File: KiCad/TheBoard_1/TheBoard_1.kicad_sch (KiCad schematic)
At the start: 27 parts, among them U1 TL431D, U2 TL431D, U4 TL431D, U5 TL431D

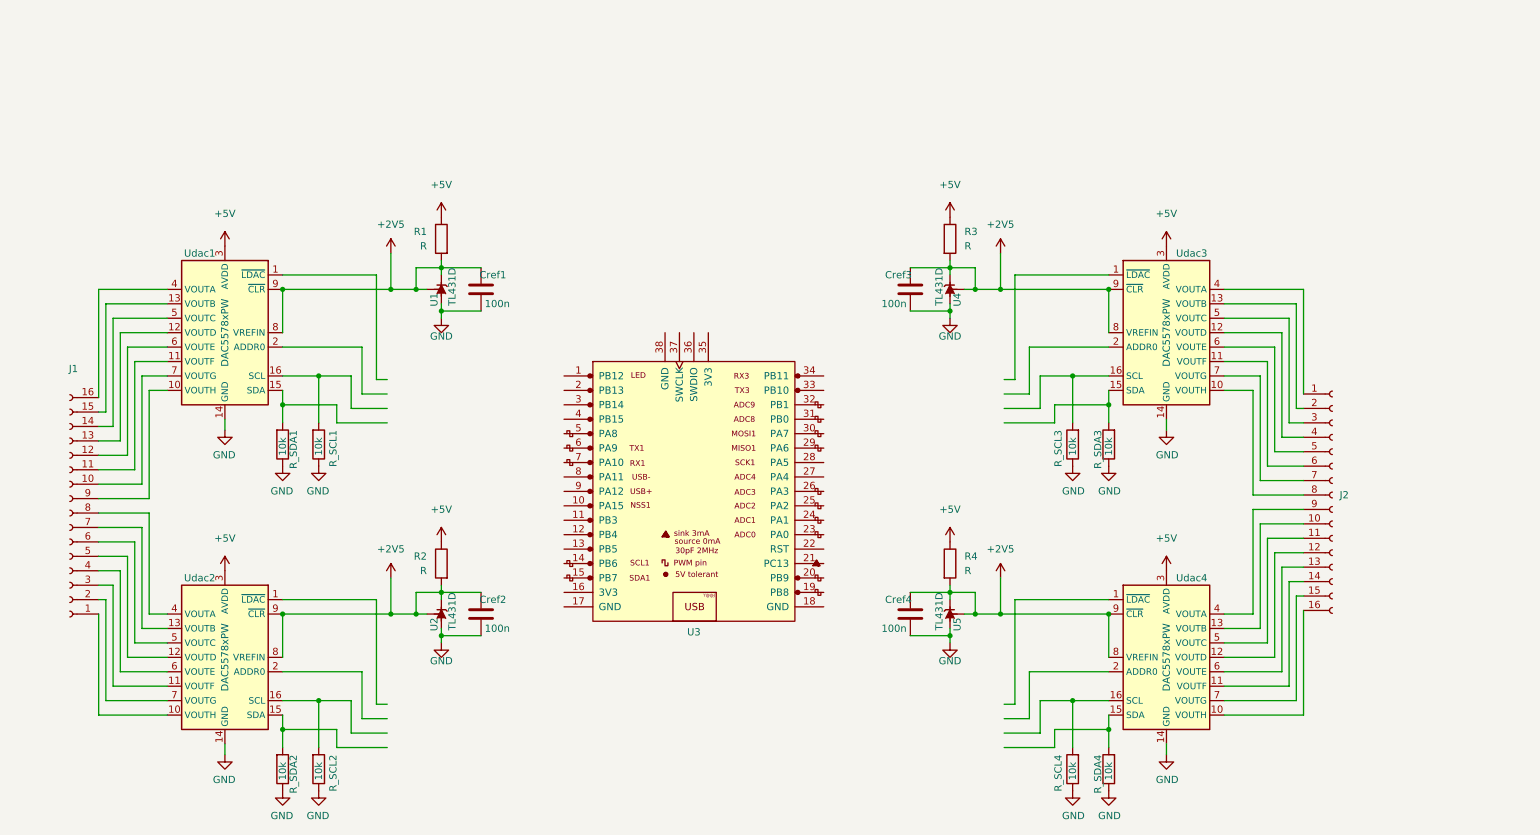
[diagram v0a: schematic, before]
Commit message: progress
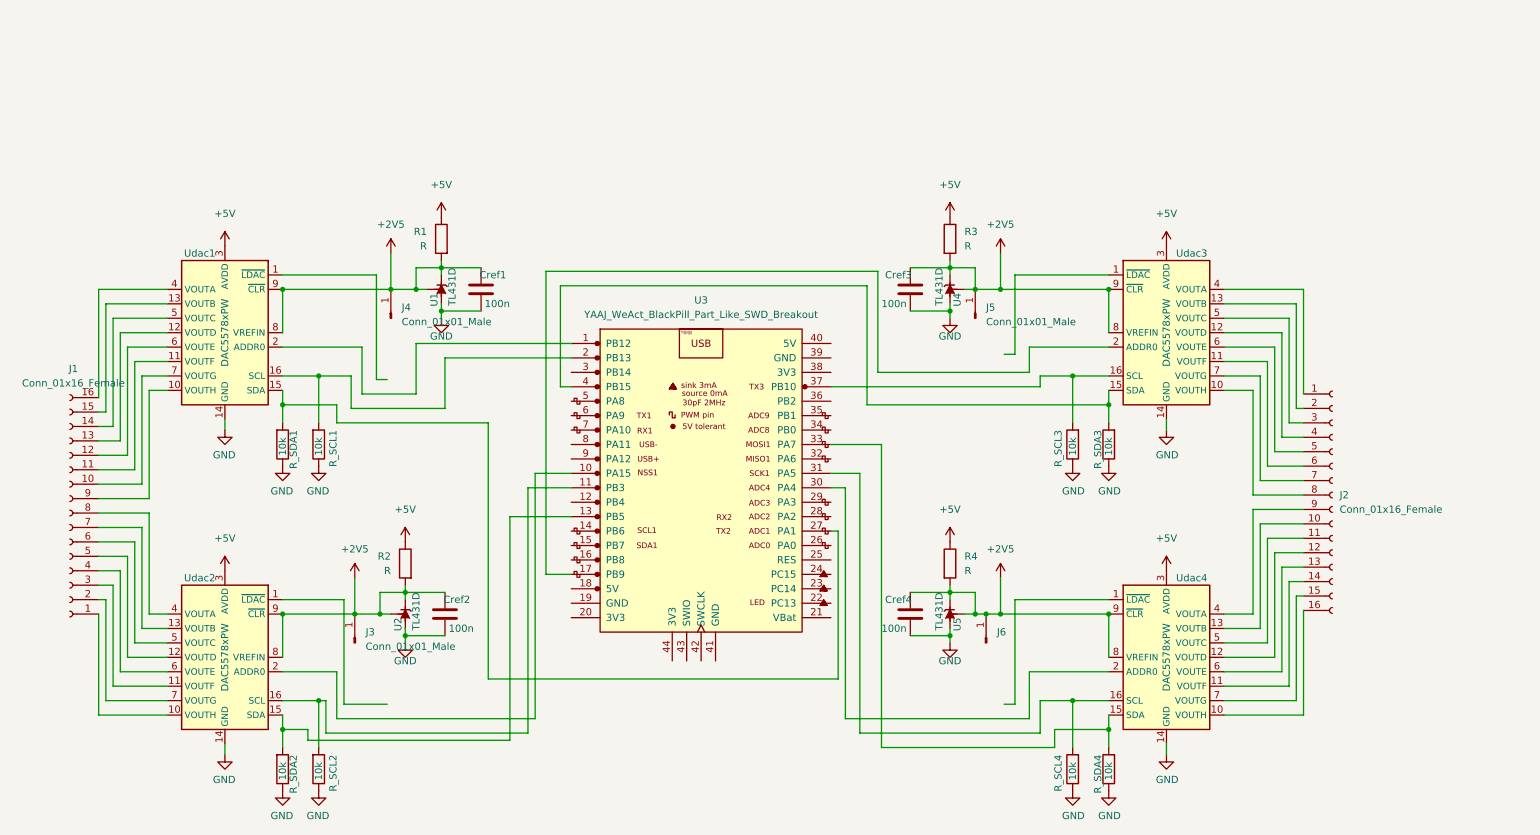
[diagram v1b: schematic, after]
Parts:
- removed U3: (no value), symbol YAAJ_BlackPill_Part_Like_SWD_Breakout:YAAJ_BlackPill_Part_Like_SWD_Breakout
- added J3, J4, J5: Conn_01x01_Male, symbol Connector:Conn_01x01_Male
- added J6: (no value), symbol Connector:Conn_01x01_Male
- added U3: YAAJ_WeAct_BlackPill_Part_Like_SWD_Breakout, symbol YAAJ_WeAct_BlackPill_Part_Like_SWD_Breakout:YAAJ_WeAct_BlackPill_Part_Like_SWD_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
- J1, J2: value (none) -> Conn_01x16_Female; footprint (none) -> Connector_PinHeader_2.54mm:PinHeader_1x16_P2.54mm_Vertical
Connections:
- net +2V5: now also J3.1 (Pin_1), J4.1 (Pin_1), J5.1 (Pin_1), J6.1 (Pin_1)
- net at R_SCL4.2, Udac4.16 (SCL): now also U3.31 (PA5)
- net at R_SCL2.2, Udac2.16 (SCL): now also U3.11 (PB3)
- net at R_SDA3.2, Udac3.15 (SDA): now also U3.4 (PB15)
- net at R_SCL3.2, Udac3.16 (SCL): now also U3.37 (PB10)
- net at Udac3.2 (ADDR0): now also U3.17 (PB9)
- net at R_SCL1.2, Udac1.16 (SCL): now also U3.2 (PB13)
- net at R_SDA2.2, Udac2.15 (SDA): now also U3.13 (PB5)
- net at Udac2.2 (ADDR0): now also U3.10 (PA15)
- net at R_SDA1.2, Udac1.15 (SDA): now also U3.27 (PA1)
- net at R_SDA4.2, Udac4.15 (SDA): now also U3.33 (PA7)
- net at Udac4.2 (ADDR0): now also U3.30 (PA4)
- net at Udac1.2 (ADDR0): now also U3.1 (PB12)
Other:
- moved on the sheet: Cref2, R2, U2

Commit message: progress
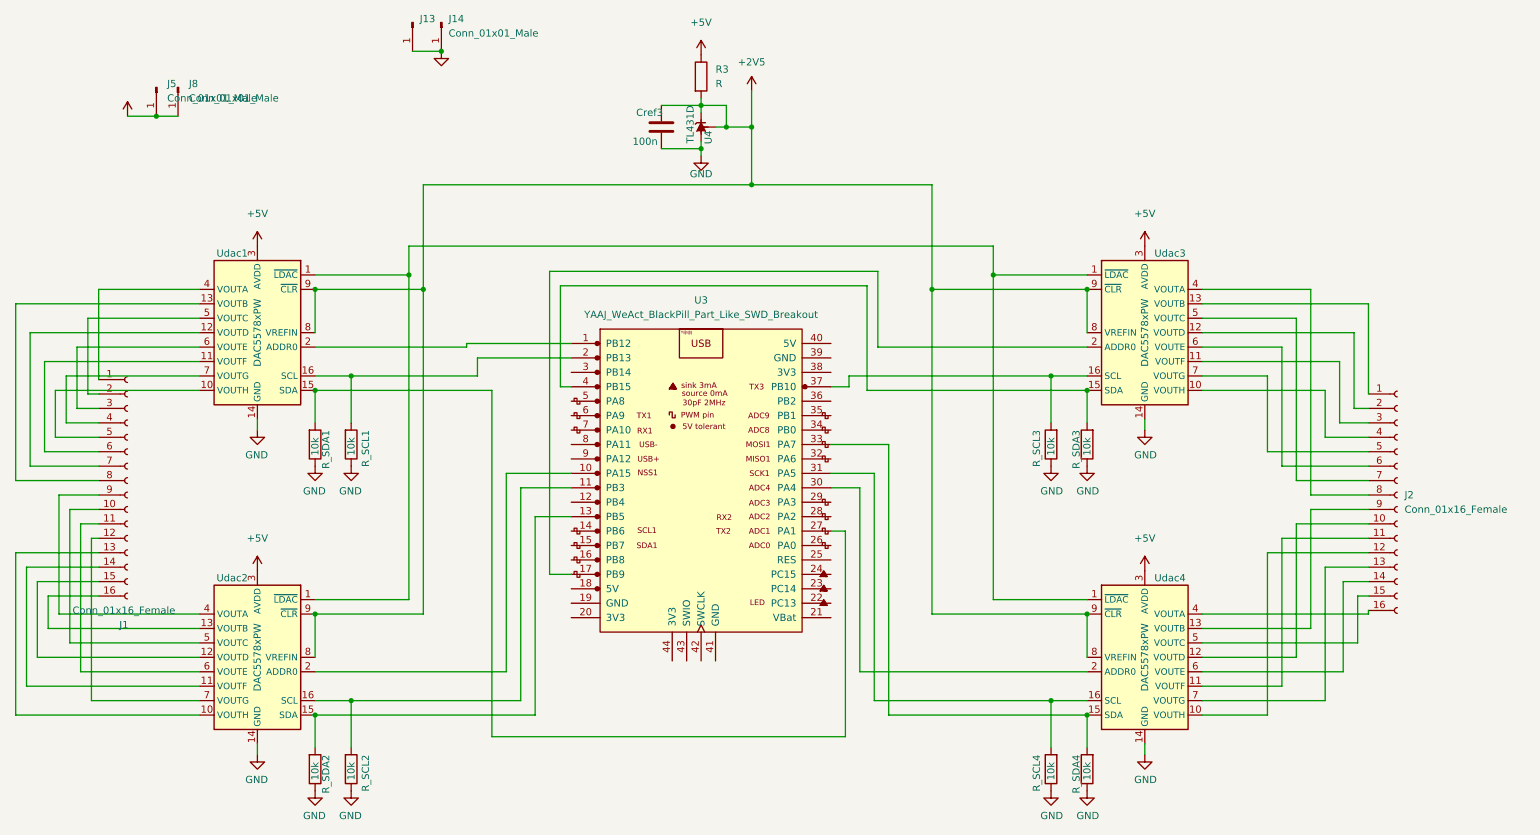
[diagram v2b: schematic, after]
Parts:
- removed Cref1, Cref2, Cref4: 100n, Capacitor_THT:C_Disc_D5.0mm_W2.5mm_P2.50mm, symbol Device:C
- removed J3, J4: Conn_01x01_Male, symbol Connector:Conn_01x01_Male
- removed J6: (no value), symbol Connector:Conn_01x01_Male
- removed R1, R2, R4: R, Resistor_THT:R_Axial_DIN0207_L6.3mm_D2.5mm_P10.16mm_Horizontal, symbol Device:R
- removed U1, U2, U5: TL431D, Package_SO:SOIC-8_3.9x4.9mm_P1.27mm, symbol Reference_Voltage:TL431D
- added J13: (no value), symbol Connector:Conn_01x01_Male
- added J14, J8: Conn_01x01_Male, symbol Connector:Conn_01x01_Male
- U3: footprint (none) -> Footprints:YAAJ_WeAct_BlackPill_SWD_2
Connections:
- net +2V5: no longer J5.1 (Pin_1)
- net +5V: now also J5.1 (Pin_1), J8.1 (Pin_1)
- net GND: now also J13.1 (Pin_1), J14.1 (Pin_1)
- net at Udac3.1 (~{LDAC}): now also Udac1.1 (~{LDAC}), Udac2.1 (~{LDAC}), Udac4.1 (~{LDAC})
- net at Udac3.10 (VOUTH): now also J2.4 (Pin_4); no longer J2.8 (Pin_8)
- net at Udac3.11 (VOUTF): now also J2.3 (Pin_3); no longer J2.6 (Pin_6)
- net at Udac3.12 (VOUTD): now also J2.2 (Pin_2); no longer J2.4 (Pin_4)
- net at Udac3.13 (VOUTB): now also J2.1 (Pin_1); no longer J2.2 (Pin_2)
- net at Udac3.4 (VOUTA): now also J2.8 (Pin_8); no longer J2.1 (Pin_1)
- net at Udac3.5 (VOUTC): now also J2.7 (Pin_7); no longer J2.3 (Pin_3)
- net at Udac3.6 (VOUTE): now also J2.6 (Pin_6); no longer J2.5 (Pin_5)
- net at Udac3.7 (VOUTG): now also J2.5 (Pin_5); no longer J2.7 (Pin_7)
- net at Udac2.10 (VOUTH): now also J1.13 (Pin_13); no longer J1.1 (Pin_1)
- net at Udac2.11 (VOUTF): now also J1.14 (Pin_14); no longer J1.3 (Pin_3)
- net at Udac2.12 (VOUTD): now also J1.15 (Pin_15); no longer J1.5 (Pin_5)
- net at Udac2.13 (VOUTB): now also J1.16 (Pin_16); no longer J1.7 (Pin_7)
- net at Udac2.4 (VOUTA): now also J1.9 (Pin_9); no longer J1.8 (Pin_8)
- net at Udac2.5 (VOUTC): now also J1.10 (Pin_10); no longer J1.6 (Pin_6)
- net at Udac2.6 (VOUTE): now also J1.11 (Pin_11); no longer J1.4 (Pin_4)
- net at Udac2.7 (VOUTG): now also J1.12 (Pin_12); no longer J1.2 (Pin_2)
- net at J2.10 (Pin_10): now also Udac4.12 (VOUTD); no longer Udac4.13 (VOUTB)
- net at J2.11 (Pin_11): now also Udac4.11 (VOUTF); no longer Udac4.5 (VOUTC)
- net at J2.12 (Pin_12): now also Udac4.10 (VOUTH); no longer Udac4.12 (VOUTD)
- net at J2.13 (Pin_13): now also Udac4.7 (VOUTG); no longer Udac4.6 (VOUTE)
- net at J2.14 (Pin_14): now also Udac4.6 (VOUTE); no longer Udac4.11 (VOUTF)
- net at J2.15 (Pin_15): now also Udac4.5 (VOUTC); no longer Udac4.7 (VOUTG)
- net at J2.16 (Pin_16): now also Udac4.4 (VOUTA); no longer Udac4.10 (VOUTH)
- net at J2.9 (Pin_9): now also Udac4.13 (VOUTB); no longer Udac4.4 (VOUTA)
- net at Udac1.10 (VOUTH): now also J1.5 (Pin_5); no longer J1.9 (Pin_9)
- net at Udac1.11 (VOUTF): now also J1.6 (Pin_6); no longer J1.11 (Pin_11)
- net at Udac1.12 (VOUTD): now also J1.7 (Pin_7); no longer J1.13 (Pin_13)
- net at Udac1.13 (VOUTB): now also J1.8 (Pin_8); no longer J1.15 (Pin_15)
- net at Udac1.4 (VOUTA): now also J1.1 (Pin_1); no longer J1.16 (Pin_16)
- net at Udac1.5 (VOUTC): now also J1.2 (Pin_2); no longer J1.14 (Pin_14)
- net at Udac1.6 (VOUTE): now also J1.3 (Pin_3); no longer J1.12 (Pin_12)
- net at Udac1.7 (VOUTG): now also J1.4 (Pin_4); no longer J1.10 (Pin_10)
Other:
- moved on the sheet: Cref3, J1, J2, R3, R_SCL1, R_SCL2, R_SCL3, R_SCL4, R_SDA1, R_SDA2, R_SDA3, R_SDA4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

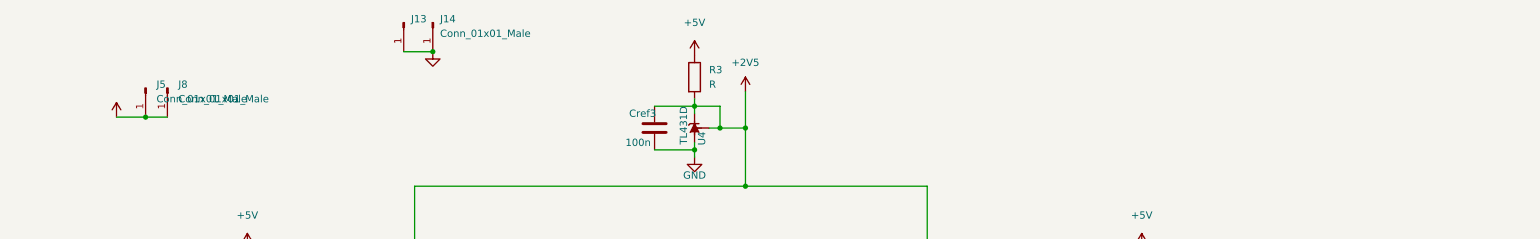
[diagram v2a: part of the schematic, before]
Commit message: progress - almost done
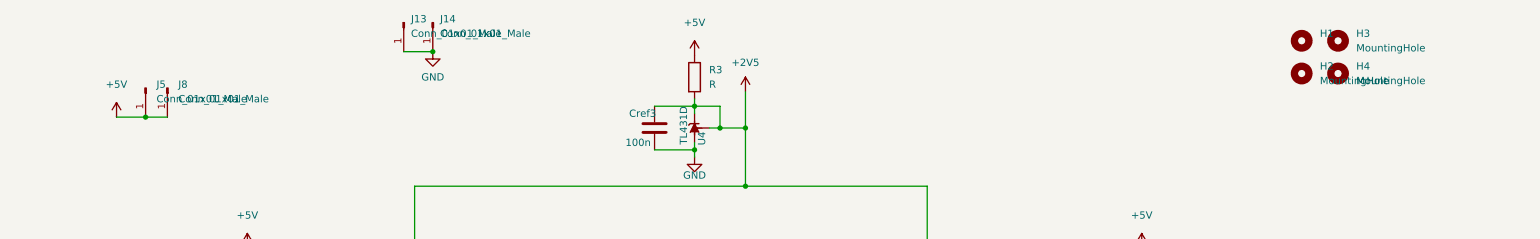
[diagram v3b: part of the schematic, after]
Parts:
- added H1: (no value), symbol Mechanical:MountingHole
- added H2, H3, H4: MountingHole, symbol Mechanical:MountingHole
- J13: value (none) -> Conn_01x01_Male; footprint (none) -> Connector_PinHeader_2.54mm:PinHeader_1x01_P2.54mm_Vertical
- J14, J5, J8: footprint (none) -> Connector_PinHeader_2.54mm:PinHeader_1x01_P2.54mm_Vertical
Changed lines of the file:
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@@
       (effects (font (size 1.27 1.27)) (justify left))
     )
-    (property "Footprint" "" (id 2) (at 52.705 31.115 0)
+    (property "Footprint" "Connector_PinHeader_2.54mm:PinHeader_1x01_P2.54mm_Vertical" (id 2) (at 52.705 31.115 0)
       (effects (font (size 1.27 1.27)) hide)
     )
@@
       (effects (font (size 1.27 1.27)) (justify left))
     )
-    (property "Footprint" "" (id 2) (at 102.87 19.685 0)
+    (property "Footprint" "Connector_PinHeader_2.54mm:PinHeader_1x01_P2.54mm_Vertical" (id 2) (at 102.87 19.685 0)
       (effects (font (size 1.27 1.27)) hide)
     )
@@
       (effects (font (size 1.27 1.27)) (justify left))
     )
-    (property "Value" "" (id 1) (at 99.06 21.5899 90)
-      (effects (font (size 1.27 1.27)) (justify left))
-    )
-    (property "Footprint" "" (id 2) (at 97.79 19.685 0)
+    (property "Value" "Conn_01x01_Male" (id 1) (at 99.06 21.5899 90)
+      (effects (font (size 1.27 1.27)) (justify left))
+    )
+    (property "Footprint" "Connector_PinHeader_2.54mm:PinHeader_1x01_P2.54mm_Vertical" (id 2) (at 97.79 19.685 0)
       (effects (font (size 1.27 1.27)) hide)
     )
@@
     (pin "1")
     (pin "2")
+  )
+  (symbol (lib_id "Mechanical:MountingHole") (at 260.985 22.86 0) (unit 1)
+    (in_bom yes) (on_board yes) (fields_autoplaced)
+    (property "Reference" "H3" (id 0) (at 264.16 21.5899 0)
+      (effects (font (size 1.27 1.27)) (justify left))
+    )
+    (property "Value" "MountingHole" (id 1) (at 264.16 24.1299 0)
+      (effects (font (size 1.27 1.27)) (justify left))
+    )
+    (property "Footprint" "" (id 2) (at 260.985 22.86 0)
+      (effects (font (size 1.27 1.27)) hide)
+    )
+    (property "Datasheet" "~" (id 3) (at 260.985 22.86 0)
+      (effects (font (size 1.27 1.27)) hide)
+    )
   )
   (symbol (lib_id "YAAJ_WeAct_BlackPill_Part_Like_SWD_Breakout:YAAJ_WeAct_BlackPill_Part_Like_SWD_Breakout") (at 148.59 99.06 0) (unit 1)
@@
       (effects (font (size 1.27 1.27)) hide)
     )
-    (property "Value" "" (id 1) (at 47.625 30.48 0))
+    (property "Value" "+5V" (id 1) (at 47.625 30.48 0))
     (property "Footprint" "" (id 2) (at 47.625 36.195 0)
       (effects (font (size 1.27 1.27)) hide)
@@
     (pin "2")
   )
+  (symbol (lib_id "Mechanical:MountingHole") (at 254.635 28.575 0) (unit 1)
+    (in_bom yes) (on_board yes) (fields_autoplaced)
+    (property "Reference" "H2" (id 0) (at 257.81 27.3049 0)
+      (effects (font (size 1.27 1.27)) (justify left))
+    )
+    (property "Value" "MountingHole" (id 1) (at 257.81 29.8449 0)
+      (effects (font (size 1.27 1.27)) (justify left))
+    )
+    (property "Footprint" "" (id 2) (at 254.635 28.575 0)
+      (effects (font (size 1.27 1.27)) hide)
+    )
+    (property "Datasheet" "~" (id 3) (at 254.635 28.575 0)
+      (effects (font (size 1.27 1.27)) hide)
+    )
+  )
   (symbol (lib_id "power:GND") (at 102.87 24.765 0) (unit 1)
     (in_bom yes) (on_board yes) (fields_autoplaced)
@@
       (effects (font (size 1.27 1.27)) hide)
     )
-    (property "Value" "" (id 1) (at 102.87 29.21 0))
+    (property "Value" "GND" (id 1) (at 102.87 29.21 0))
     (property "Footprint" "" (id 2) (at 102.87 24.765 0)
       (effects (font (size 1.27 1.27)) hide)
@@
     (pin "2")
   )
+  (symbol (lib_id "Mechanical:MountingHole") (at 260.985 28.575 0) (unit 1)
+    (in_bom yes) (on_board yes) (fields_autoplaced)
+    (property "Reference" "H4" (id 0) (at 264.16 27.3049 0)
+      (effects (font (size 1.27 1.27)) (justify left))
+    )
+    (property "Value" "MountingHole" (id 1) (at 264.16 29.8449 0)
+      (effects (font (size 1.27 1.27)) (justify left))
+    )
+    (property "Footprint" "" (id 2) (at 260.985 28.575 0)
+      (effects (font (size 1.27 1.27)) hide)
+    )
+    (property "Datasheet" "~" (id 3) (at 260.985 28.575 0)
+      (effects (font (size 1.27 1.27)) hide)
+    )
+  )
   (symbol (lib_id "Connector:Conn_01x01_Male") (at 56.515 31.115 270) (unit 1)
     (in_bom yes) (on_board yes) (fields_autoplaced)
@@
       (effects (font (size 1.27 1.27)) (justify left))
     )
-    (property "Footprint" "" (id 2) (at 56.515 31.115 0)
+    (property "Footprint" "Connector_PinHeader_2.54mm:PinHeader_1x01_P2.54mm_Vertical" (id 2) (at 56.515 31.115 0)
       (effects (font (size 1.27 1.27)) hide)
     )
@@
     (pin "9")
   )
+  (symbol (lib_id "Mechanical:MountingHole") (at 254.635 22.86 0) (unit 1)
+    (in_bom yes) (on_board yes) (fields_autoplaced)
+    (property "Reference" "H1" (id 0) (at 257.81 21.5899 0)
+      (effects (font (size 1.27 1.27)) (justify left))
+    )
+    (property "Value" "" (id 1) (at 257.81 24.1299 0)
+      (effects (font (size 1.27 1.27)) (justify left))
+    )
+    (property "Footprint" "" (id 2) (at 254.635 22.86 0)
+      (effects (font (size 1.27 1.27)) hide)
+    )
+    (property "Datasheet" "~" (id 3) (at 254.635 22.86 0)
+      (effects (font (size 1.27 1.27)) hide)
+    )
+  )
   (symbol (lib_id "Connector:Conn_01x16_Female") (at 47.625 100.33 0) (unit 1)
     (in_bom yes) (on_board yes) (fields_autoplaced)
@@
       (reference "Cref3") (unit 1) (value "100n") (footprint "Capacitor_THT:C_Disc_D5.0mm_W2.5mm_P2.50mm")
     )
+    (path "/e873deca-9d09-405a-95a4-80d6995b5991"
+      (reference "H1") (unit 1) (value "MountingHole") (footprint "MountingHole:MountingHole_3mm")
+    )
+    (path "/adc35284-b1a5-4a4f-9d67-d284094a133d"
+      (reference "H2") (unit 1) (value "MountingHole") (footprint "MountingHole:MountingHole_3mm")
+    )
+    (path "/991f0149-2129-43f5-b512-8a3a239e334e"
+      (reference "H3") (unit 1) (value "MountingHole") (footprint "MountingHole:MountingHole_3mm")
+    )
+    (path "/bb4a7035-f90e-4d07-853b-36c6c31e27d3"
+      (reference "H4") (unit 1) (value "MountingHole") (footprint "MountingHole:MountingHole_3mm")
+    )
     (path "/e9eb63c6-f195-43e4-bcf3-d789bacf3bde"
